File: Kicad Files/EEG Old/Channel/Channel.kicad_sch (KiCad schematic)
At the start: 28 parts, among them J1 Conn_01x02_Pin, J2 Conn_01x07_Pin, U1 INA823, U2 LF356N, U3 LF356N, U4 LF356N, U5 LF356N, U6 MCP4161

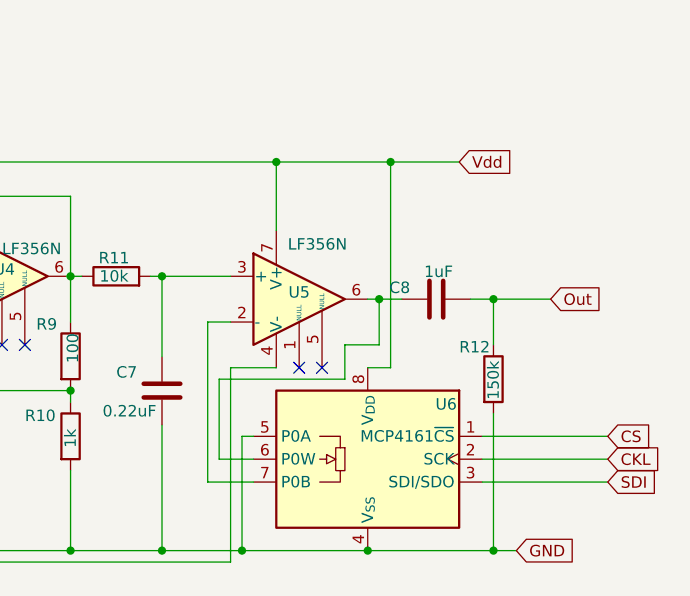
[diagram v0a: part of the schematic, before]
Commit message: Corrections in EEG
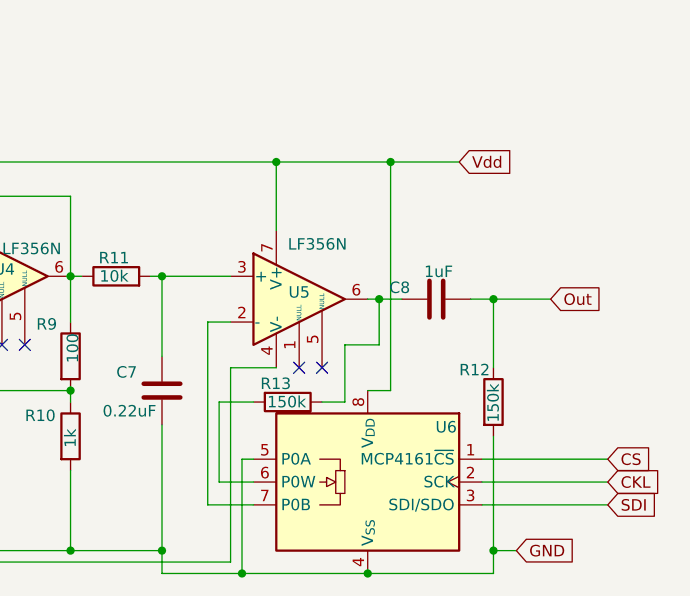
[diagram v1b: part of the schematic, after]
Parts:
- added R13: 150k, Resistor_SMD:R_0402_1005Metric_Pad0.72x0.64mm_HandSolder, symbol Device:R
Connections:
- net at C8.1, U5.6: now also R13.1; no longer U6.6 (P0W)
- new net: R13.2, U6.6 (P0W)
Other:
- moved on the sheet: R12, U6
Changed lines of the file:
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@@
 	)
 	(junction
-		(at 213.36 115.57)
+		(at 213.36 118.11)
 		(diameter 0)
 		(color 0 0 0 0)
@@
 	)
 	(junction
-		(at 199.39 115.57)
+		(at 199.39 118.11)
 		(diameter 0)
 		(color 0 0 0 0)
@@
 	(wire
 		(pts
+			(xy 190.5 118.11) (xy 190.5 115.57)
+		)
+		(stroke
+			(width 0)
+			(type default)
+		)
+	)
+	(wire
+		(pts
 			(xy 59.69 116.84) (xy 86.36 116.84)
 		)
@@
 	(wire
 		(pts
-			(xy 215.9 95.25) (xy 213.36 95.25)
+			(xy 215.9 97.79) (xy 213.36 97.79)
+		)
+		(stroke
+			(width 0)
+			(type default)
+		)
+	)
+	(wire
+		(pts
+			(xy 227.33 118.11) (xy 227.33 115.57)
 		)
 		(stroke
@@
 	(wire
 		(pts
-			(xy 199.39 102.87) (xy 199.39 115.57)
+			(xy 199.39 105.41) (xy 199.39 118.11)
 		)
 		(stroke
@@
 	(wire
 		(pts
-			(xy 190.5 115.57) (xy 199.39 115.57)
+			(xy 190.5 118.11) (xy 199.39 118.11)
 		)
 		(stroke
@@
 	(wire
 		(pts
+			(xy 196.85 99.06) (xy 200.66 99.06)
+		)
+		(stroke
+			(width 0)
+			(type default)
+		)
+	)
+	(wire
+		(pts
 			(xy 110.49 101.6) (xy 110.49 104.14)
 		)
@@
 	(wire
 		(pts
-			(xy 195.58 107.95) (xy 195.58 90.17)
+			(xy 195.58 110.49) (xy 195.58 90.17)
 		)
 		(stroke
@@
 	(wire
 		(pts
-			(xy 226.06 102.87) (xy 240.03 102.87)
+			(xy 226.06 105.41) (xy 240.03 105.41)
 		)
 		(stroke
@@
 	(wire
 		(pts
-			(xy 196.85 105.41) (xy 196.85 96.52)
+			(xy 196.85 107.95) (xy 196.85 99.06)
 		)
 		(stroke
@@
 	(wire
 		(pts
-			(xy 226.06 107.95) (xy 240.03 107.95)
+			(xy 226.06 110.49) (xy 240.03 110.49)
 		)
 		(stroke
@@
 	(wire
 		(pts
-			(xy 226.06 105.41) (xy 240.03 105.41)
+			(xy 226.06 107.95) (xy 240.03 107.95)
 		)
 		(stroke
@@
 	(wire
 		(pts
-			(xy 227.33 87.63) (xy 227.33 92.71)
+			(xy 227.33 87.63) (xy 227.33 95.25)
 		)
 		(stroke
@@
 	(wire
 		(pts
-			(xy 200.66 105.41) (xy 196.85 105.41)
+			(xy 200.66 107.95) (xy 196.85 107.95)
 		)
 		(stroke
@@
 	(wire
 		(pts
-			(xy 213.36 115.57) (xy 227.33 115.57)
+			(xy 213.36 118.11) (xy 227.33 118.11)
 		)
 		(stroke
@@
 	(wire
 		(pts
-			(xy 199.39 115.57) (xy 213.36 115.57)
+			(xy 199.39 118.11) (xy 213.36 118.11)
 		)
 		(stroke
@@
 	(wire
 		(pts
-			(xy 200.66 102.87) (xy 199.39 102.87)
+			(xy 200.66 105.41) (xy 199.39 105.41)
 		)
 		(stroke
@@
 	(wire
 		(pts
-			(xy 210.82 96.52) (xy 210.82 92.71)
+			(xy 210.82 99.06) (xy 210.82 92.71)
 		)
 		(stroke
@@
 	(wire
 		(pts
-			(xy 227.33 100.33) (xy 227.33 115.57)
+			(xy 227.33 102.87) (xy 227.33 115.57)
 		)
 		(stroke
@@
 	(wire
 		(pts
-			(xy 215.9 72.39) (xy 215.9 95.25)
+			(xy 215.9 72.39) (xy 215.9 97.79)
 		)
 		(stroke
@@
 	(wire
 		(pts
-			(xy 195.58 107.95) (xy 200.66 107.95)
+			(xy 195.58 110.49) (xy 200.66 110.49)
 		)
 		(stroke
@@
 	(wire
 		(pts
-			(xy 196.85 96.52) (xy 210.82 96.52)
+			(xy 137.16 72.39) (xy 125.73 72.39)
 		)
 		(stroke
@@
 	(wire
 		(pts
-			(xy 137.16 72.39) (xy 125.73 72.39)
+			(xy 190.5 85.09) (xy 190.5 93.98)
 		)
 		(stroke
@@
 	(wire
 		(pts
-			(xy 190.5 85.09) (xy 190.5 93.98)
+			(xy 116.84 96.52) (xy 116.84 116.84)
 		)
 		(stroke
@@
 	(wire
 		(pts
-			(xy 116.84 96.52) (xy 116.84 116.84)
+			(xy 76.2 83.82) (xy 78.74 83.82)
 		)
 		(stroke
@@
 	(wire
 		(pts
-			(xy 76.2 83.82) (xy 78.74 83.82)
+			(xy 72.39 85.09) (xy 78.74 85.09)
 		)
 		(stroke
@@
 	(wire
 		(pts
-			(xy 72.39 85.09) (xy 78.74 85.09)
+			(xy 217.17 87.63) (xy 214.63 87.63)
 		)
 		(stroke
@@
 	(wire
 		(pts
-			(xy 217.17 87.63) (xy 214.63 87.63)
+			(xy 208.28 99.06) (xy 210.82 99.06)
 		)
 		(stroke
@@
 	(global_label "CKL"
 		(shape input)
-		(at 240.03 105.41 0)
+		(at 240.03 107.95 0)
 		(fields_autoplaced yes)
 		(effects
@@
 		)
 		(property "Intersheetrefs" "${INTERSHEET_REFS}"
-			(at 246.5833 105.41 0)
+			(at 246.5833 107.95 0)
 			(effects
 				(font
@@
 	(global_label "SDI"
 		(shape input)
-		(at 240.03 107.95 0)
+		(at 240.03 110.49 0)
 		(fields_autoplaced yes)
 		(effects
@@
 		)
 		(property "Intersheetrefs" "${INTERSHEET_REFS}"
-			(at 246.0995 107.95 0)
+			(at 246.0995 110.49 0)
 			(effects
 				(font
@@
 	(global_label "CS"
 		(shape input)
-		(at 240.03 102.87 0)
+		(at 240.03 105.41 0)
 		(fields_autoplaced yes)
 		(effects
@@
 		)
 		(property "Intersheetrefs" "${INTERSHEET_REFS}"
-			(at 245.4947 102.87 0)
+			(at 245.4947 105.41 0)
 			(effects
 				(font
@@
 	(symbol
 		(lib_id "Potentiometer_Digital:MCP4161-xxxx-P")
-		(at 213.36 105.41 0)
+		(at 213.36 107.95 0)
 		(mirror y)
 		(unit 1)
@@
 		(dnp no)
 		(property "Reference" "U6"
-			(at 223.266 99.314 0)
+			(at 223.266 101.854 0)
 			(effects
 				(font
@@
 		)
 		(property "Value" "MCP4161"
-			(at 220.726 102.87 0)
+			(at 220.726 105.41 0)
 			(effects
 				(font
@@
 		)
 		(property "Footprint" "Package_DIP:DIP-8_W7.62mm_Socket"
-			(at 213.36 125.73 0)
+			(at 213.36 128.27 0)
 			(effects
 				(font
@@
 		)
 		(property "Datasheet" "https://ww1.microchip.com/downloads/aemDocuments/documents/OTH/ProductDocuments/DataSheets/22059b.pdf"
-			(at 213.36 128.27 0)
+			(at 213.36 130.81 0)
 			(effects
 				(font
@@
 		)
 		(property "Description" "Single Digital Potentiometer, SPI interface, 257 taps, 5/10/50/100 kohm, non-volatile memory"
-			(at 213.36 130.81 0)
+			(at 213.36 133.35 0)
 			(effects
 				(font
@@
 	(symbol
 		(lib_id "Device:R")
-		(at 227.33 96.52 0)
+		(at 227.33 99.06 0)
 		(unit 1)
 		(exclude_from_sim no)
@@
 		(dnp no)
 		(property "Reference" "R12"
-			(at 223.52 92.964 0)
+			(at 223.52 95.504 0)
 			(effects
 				(font
@@
 		)
 		(property "Value" "150k"
-			(at 227.33 98.806 90)
+			(at 227.33 101.346 90)
 			(effects
 				(font
@@
 		)
 		(property "Footprint" "Resistor_SMD:R_0402_1005Metric_Pad0.72x0.64mm_HandSolder"
-			(at 225.552 96.52 90)
+			(at 225.552 99.06 90)
 			(effects
 				(font
@@
 		)
 		(property "Datasheet" "~"
-			(at 227.33 96.52 0)
+			(at 227.33 99.06 0)
 			(effects
 				(font
@@
 		)
 		(property "Description" "Resistor"
-			(at 227.33 96.52 0)
+			(at 227.33 99.06 0)
 			(effects
 				(font
@@
 					(unit 1)
 				)
+			)
+		)
+	)
+	(symbol
+		(lib_id "Device:R")
+		(at 204.47 99.06 270)
+		(unit 1)
+		(exclude_from_sim no)
+		(in_bom yes)
+		(on_board yes)
+		(dnp no)
+		(property "Reference" "R13"
+			(at 201.422 97.028 90)
+			(effects
+				(font
+					(size 1.27 1.27)
+				)
+				(justify left)
+			)
+		)
+		(property "Value" "150k"
+			(at 202.184 99.06 90)
+			(effects
+				(font
+					(size 1.27 1.27)
+				)
+				(justify left)
+			)
+		)
+		(property "Footprint" "Resistor_SMD:R_0402_1005Metric_Pad0.72x0.64mm_HandSolder"
+			(at 204.47 97.282 90)
+			(effects
+				(font
+					(size 1.27 1.27)
+				)
+				(hide yes)
+			)
+		)
+		(property "Datasheet" "~"
+			(at 204.47 99.06 0)
+			(effects
+				(font
+					(size 1.27 1.27)
+				)
+				(hide yes)
+			)
+		)
+		(property "Description" "Resistor"
+			(at 204.47 99.06 0)
+			(effects
+				(font
+					(size 1.27 1.27)
+				)
+				(hide yes)
+			)
+		)
+		(pin "2"
+		)
+		(pin "1"
+		)
+		(instances
+			(project "Channel"
+				(path "/b19dd3fd-f087-41ca-af79-313d90094b00"
+					(reference "R13")
+					(unit 1)
+				)
